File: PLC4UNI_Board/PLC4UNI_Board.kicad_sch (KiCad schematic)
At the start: 8 parts, among them J1 Screw_Terminal_01x04, J2 Screw_Terminal_01x05, J3 Screw_Terminal_01x02, J4 Screw_Terminal_01x03, J5 Screw_Terminal_01x03, J6 Screw_Terminal_01x04, J7 Screw_Terminal_01x06, J8 Screw_Terminal_01x02

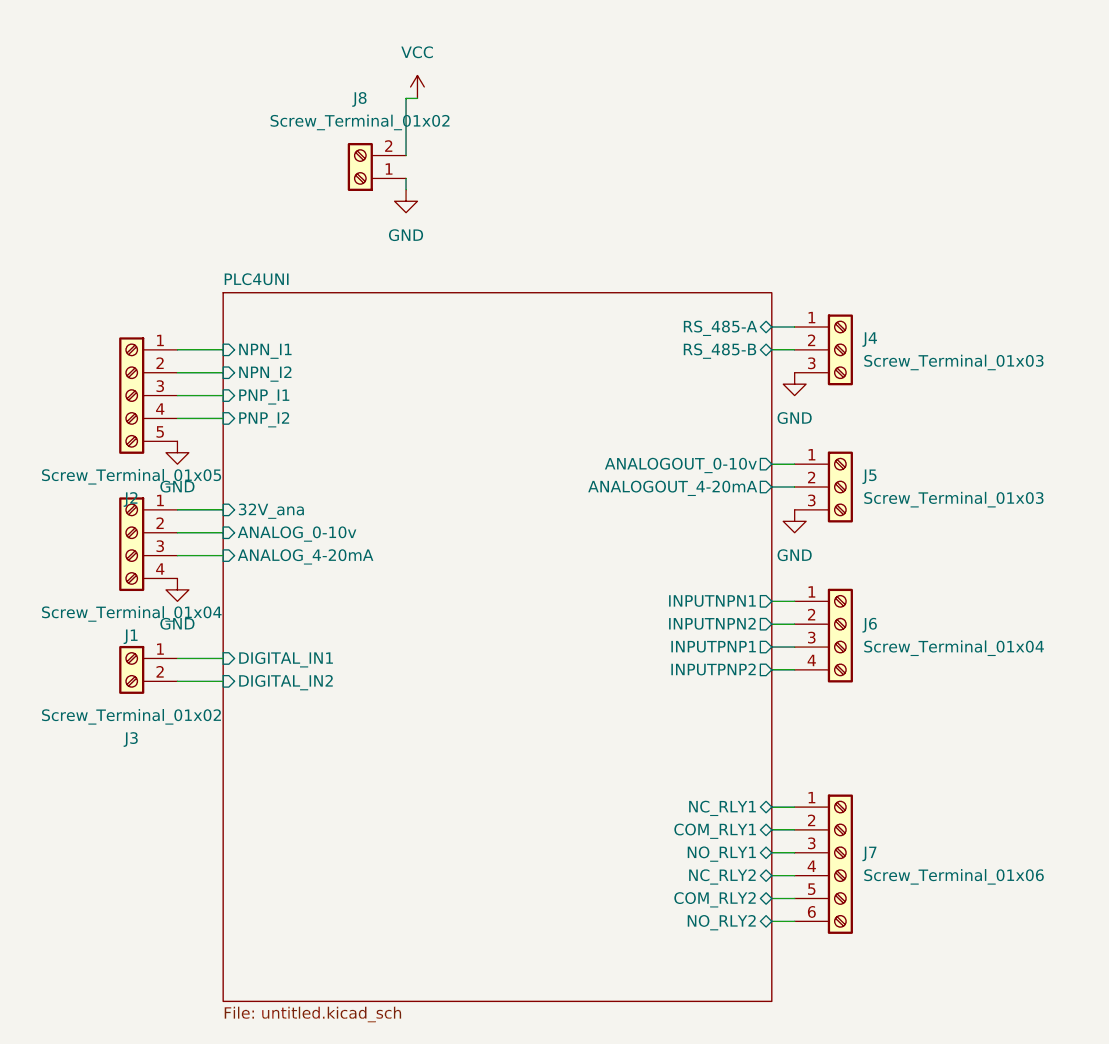
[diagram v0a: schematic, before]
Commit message: ok
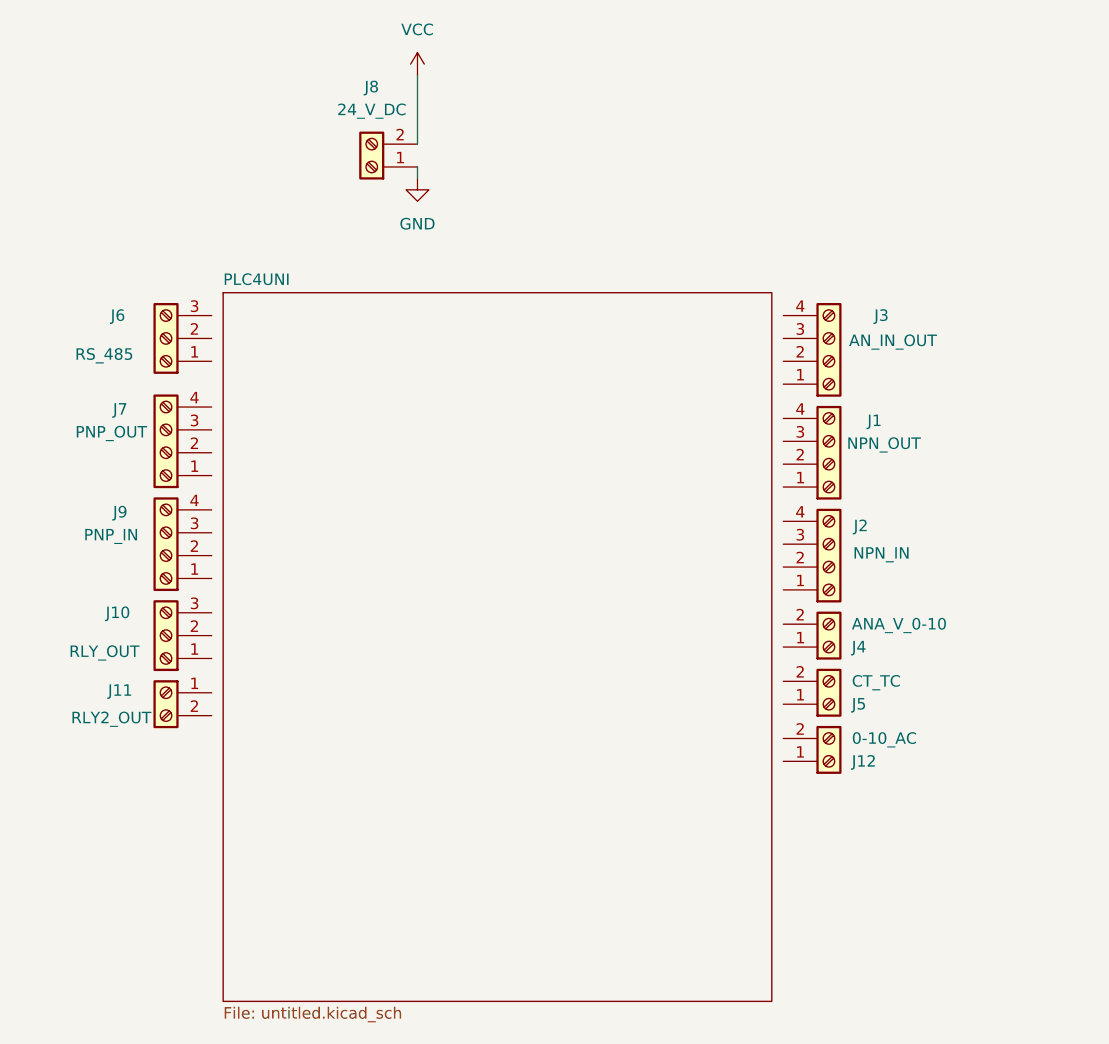
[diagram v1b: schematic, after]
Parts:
- removed J2: Screw_Terminal_01x05, symbol Connector:Screw_Terminal_01x05
- removed J3: Screw_Terminal_01x02, symbol Connector:Screw_Terminal_01x02
- removed J4, J5: Screw_Terminal_01x03, symbol Connector:Screw_Terminal_01x03
- removed J6: Screw_Terminal_01x04, symbol Connector:Screw_Terminal_01x04
- removed J7: Screw_Terminal_01x06, symbol Connector:Screw_Terminal_01x06
- added J10: RLY_OUT, symbol Connector:Screw_Terminal_01x03
- added J11: RLY2_OUT, symbol Connector:Screw_Terminal_01x02
- added J12: 0-10_AC, symbol Connector:Screw_Terminal_01x02
- added J2: NPN_IN, symbol Connector:Screw_Terminal_01x04
- added J3: AN_IN_OUT, symbol Connector:Screw_Terminal_01x04
- added J4: ANA_V_0-10, symbol Connector:Screw_Terminal_01x02
- added J5: CT_TC, symbol Connector:Screw_Terminal_01x02
- added J6: RS_485, symbol Connector:Screw_Terminal_01x03
- added J7: PNP_OUT, symbol Connector:Screw_Terminal_01x04
- added J9: PNP_IN, symbol Connector:Screw_Terminal_01x04
- J1: value Screw_Terminal_01x04 -> NPN_OUT
- J8: value Screw_Terminal_01x02 -> 24_V_DC
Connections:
- net GND: no longer J1.4 (Pin_4)
- net PLC4UNI/32V_ana: no longer names the net of J1.1 (Pin_1)
- net PLC4UNI/ANALOG_0-10v: no longer names the net of J1.2 (Pin_2)
- net PLC4UNI/ANALOG_4-20mA: no longer names the net of J1.3 (Pin_3)
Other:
- sheet PLC4UNI ports: added none; removed 32V_ana, ANALOGOUT_0-10v, ANALOGOUT_4-20mA, ANALOG_0-10v, ANALOG_4-20mA, COM_RLY1, COM_RLY2, DIGITAL_IN1, DIGITAL_IN2, INPUTNPN1, INPUTNPN2, INPUTPNP1, INPUTPNP2, NC_RLY1, NC_RLY2, NO_RLY1, NO_RLY2, NPN_I1, NPN_I2, PNP_I1, PNP_I2, RS_485-A, RS_485-B
- moved on the sheet: J8

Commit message: v.1.0.1
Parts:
- J1, J2, J9: footprint (none) -> tb-002H:TE_796683-4
- J10, J6: footprint (none) -> TB'000H:tb
- J11, J12, J4, J5, J8: footprint (none) -> tb-003H:EBBA-02-C-SS-BU
- J3, J7: footprint (none) -> TB'000H:terminal block
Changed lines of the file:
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@@
 			)
 		)
-		(property "Footprint" ""
+		(property "Footprint" "tb-003H:EBBA-02-C-SS-BU"
 			(at 132.08 58.42 0)
 			(effects
@@
 			)
 		)
-		(property "Footprint" ""
+		(property "Footprint" "TB'000H:terminal block"
 			(at 109.22 90.17 0)
 			(effects
@@
 			)
 		)
-		(property "Footprint" ""
+		(property "Footprint" "tb-003H:EBBA-02-C-SS-BU"
 			(at 182.88 124.46 0)
 			(effects
@@
 			)
 		)
-		(property "Footprint" ""
+		(property "Footprint" "tb-003H:EBBA-02-C-SS-BU"
 			(at 109.22 116.84 0)
 			(effects
@@
 			)
 		)
-		(property "Footprint" ""
+		(property "Footprint" "TB'000H:terminal block"
 			(at 182.88 80.01 0)
 			(effects
@@
 			)
 		)
-		(property "Footprint" ""
+		(property "Footprint" "TB'000H:tb"
 			(at 109.22 110.49 0)
 			(effects
@@
 			)
 		)
-		(property "Footprint" ""
+		(property "Footprint" "tb-002H:TE_796683-4"
 			(at 182.88 102.87 0)
 			(effects
@@
 			)
 		)
-		(property "Footprint" ""
+		(property "Footprint" "tb-002H:TE_796683-4"
 			(at 182.88 91.44 0)
 			(effects
@@
 			)
 		)
-		(property "Footprint" ""
+		(property "Footprint" "tb-003H:EBBA-02-C-SS-BU"
 			(at 182.88 118.11 0)
 			(effects
@@
 			)
 		)
-		(property "Footprint" ""
+		(property "Footprint" "tb-002H:TE_796683-4"
 			(at 109.22 101.6 0)
 			(effects
@@
 			)
 		)
-		(property "Footprint" ""
+		(property "Footprint" "tb-003H:EBBA-02-C-SS-BU"
 			(at 182.88 111.76 0)
 			(effects
@@
 			)
 		)
-		(property "Footprint" ""
+		(property "Footprint" "TB'000H:tb"
 			(at 109.22 77.47 0)
 			(effects
@@
 				(font
 					(size 1.27 1.27)
-				)
-				(hide yes)
+					(italic yes)
+				)
+				(hide yes)
